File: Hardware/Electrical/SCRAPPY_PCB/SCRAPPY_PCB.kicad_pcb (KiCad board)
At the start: 2 copper layers, 87.6 x 96.5 mm, 54 parts, among them J1 Screw_Terminal_01x02, J2 Conn_01x04, J3 Conn_01x03, J4 Conn_01x03, J5 Conn_01x03, J6 Conn_01x04, J7 Conn_01x04, J8 Conn_01x04, J9 Conn_01x04, Q1 PN2222A, Q2 PN2222A, Q3 PN2222A, U1 ESP32-DevBoard, U2 L7805, U3 LM324

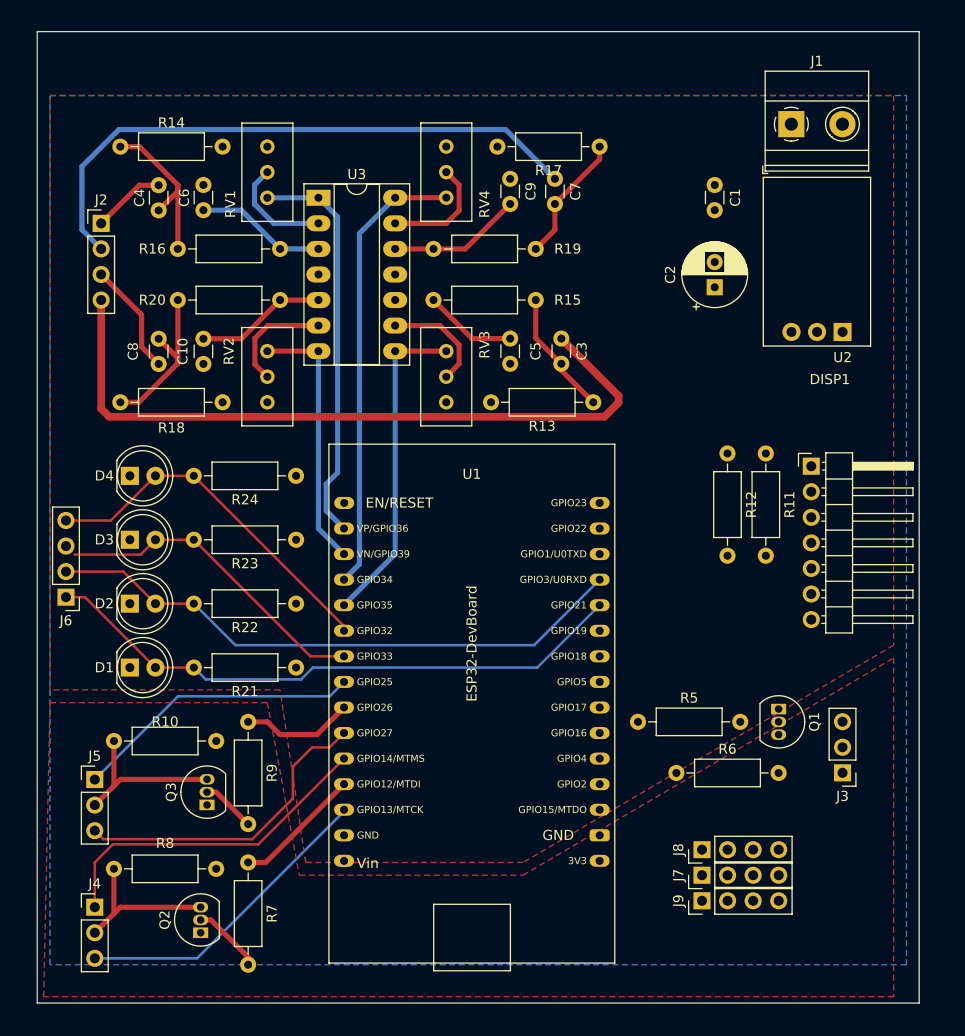
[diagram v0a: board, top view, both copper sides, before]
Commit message: Updated PCB; Ready for Manufacture
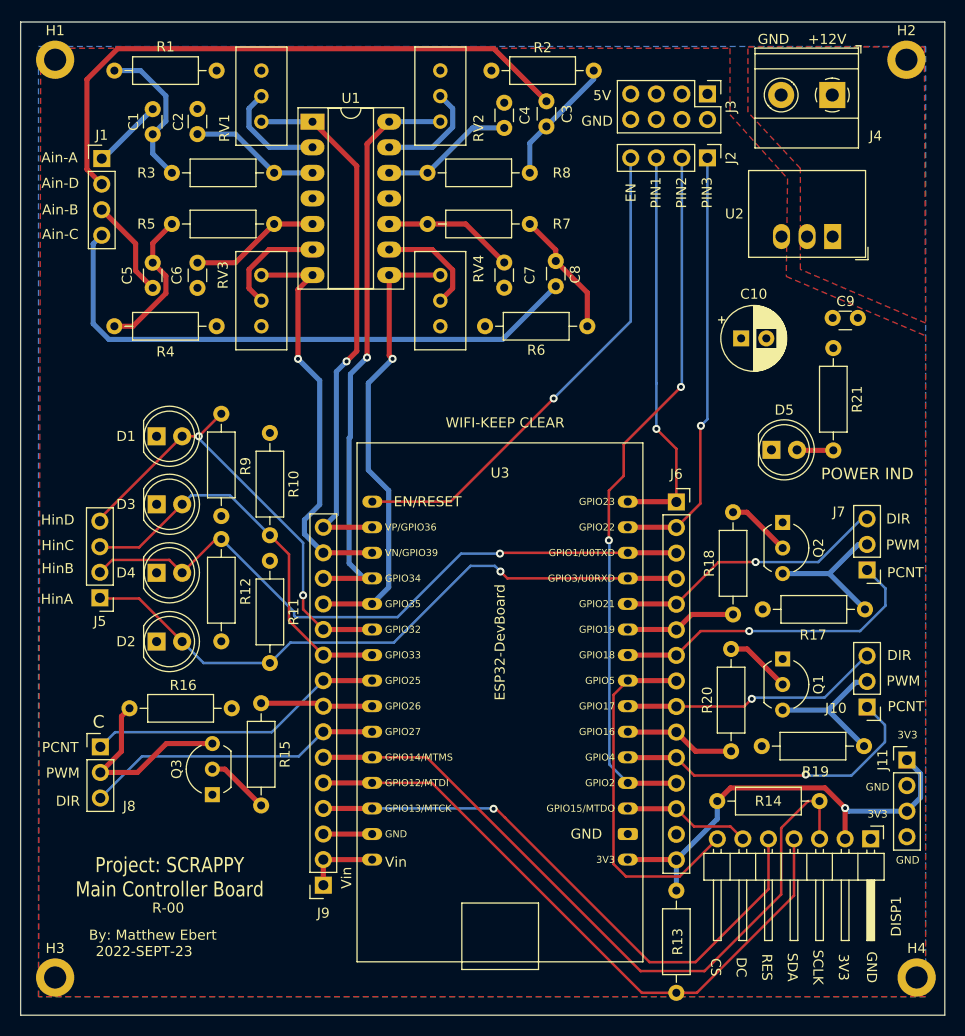
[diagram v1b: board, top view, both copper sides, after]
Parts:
- removed the J7 at (115.6, 133.3)
- added D5: LED, LED_THT:LED_D5.0mm_Clear, F.Cu at (122.5, 91.1)
- added H1: MountingHole, MountingHole:MountingHole_2.2mm_M2_DIN965_Pad, F.Cu at (51.3, 52.3)
- added H2: MountingHole, MountingHole:MountingHole_2.2mm_M2_DIN965_Pad, F.Cu at (135.9, 52.3)
- added H3: MountingHole, MountingHole:MountingHole_2.2mm_M2_DIN965_Pad, F.Cu at (51.3, 143.5)
- added H4: MountingHole, MountingHole:MountingHole_2.2mm_M2_DIN965_Pad, F.Cu at (136.9, 143.5)
- added J11: Conn_02x02_Odd_Even, Connector_PinHeader_2.54mm:PinHeader_1x04_P2.54mm_Vertical, F.Cu at (135.9, 121.9)
- added J3: Conn_02x04_Counter_Clockwise, Connector_PinHeader_2.54mm:PinHeader_2x04_P2.54mm_Vertical, F.Cu at (116.1, 55.7)
- added J6: Conn_01x15, Connector_PinSocket_2.54mm:PinSocket_1x15_P2.54mm_Vertical, F.Cu at (113.0, 96.3)
- added R21: R, Resistor_THT:R_Axial_DIN0207_L6.3mm_D2.5mm_P10.16mm_Horizontal, F.Cu at (128.6, 81.0)
- J9: value Conn_01x04 -> Conn_01x15; footprint Connector_PinHeader_2.54mm:PinHeader_1x04_P2.54mm_Vertical -> Connector_PinSocket_2.54mm:PinSocket_1x15_P2.54mm_Vertical
- Q1, Q2, Q3: footprint Package_TO_SOT_THT:TO-92_Inline -> Package_TO_SOT_THT:TO-92_Inline_Wide
- U2: footprint Converter_DCDC:Converter_DCDC_Murata_OKI-78SR_Horizontal -> Converter_DCDC:Converter_DCDC_RECOM_R-78B-2.0_THT
- moved J7 83.7 mm to (132.0, 103.0), turned to 180 degrees
- moved Q2 70.8 mm to (123.6, 98.3), turned to -90 degrees
- moved J2 68.7 mm to (116.1, 62.1), turned to -90 degrees
- moved R17 60.1 mm to (121.6, 106.9), turned to 0 degrees
- moved R18 54.1 mm to (118.7, 107.4), turned to 90 degrees
- moved R13 44.3 mm to (113.0, 134.9)
- moved J9 37.7 mm to (78.0, 134.3), turned to 180 degrees
- moved DISP1 37.5 mm to (132.3, 129.7), turned to -90 degrees
- moved R14 34.6 mm to (117.1, 126.0), turned to 0 degrees
- moved C9 19.6 mm to (131.1, 78.2), turned to 180 degrees
- moved R10 10.9 mm to (72.6, 89.4), turned to -90 degrees
- moved R11 10.9 mm to (72.6, 102.1), turned to -90 degrees
- moved R20 9.70 mm to (118.5, 121.0), turned to 90 degrees
- moved U2 9.53 mm to (128.6, 69.9)
- moved R19 8.90 mm to (121.5, 120.5)
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- renumbered C4 to C1, C2 to C10, C6 to C2, C7 to C3, C9 to C4, C8 to C5, C10 to C6, C5 to C7, C3 to C8, C1 to C9, D4 to D1, D1 to D2, D2 to D4, J2 to J1, J3 to J10, J8 to J2, J1 to J4, J6 to J5, J4 to J7, J5 to J8, R14 to R1, R23 to R10, R21 to R11, R22 to R12, R11 to R13, R12 to R14, R9 to R15, R10 to R16, R8 to R17, R7 to R18, R6 to R19, R17 to R2, R5 to R20, R16 to R3, R18 to R4, R20 to R5, R13 to R6, R15 to R7, R19 to R8, R24 to R9, RV4 to RV2, RV2 to RV3, RV3 to RV4, U3 to U1, U1 to U3
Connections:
- C9 pad 2: +12V -> +5V
- J2 pad 1: /PIN_1 -> /PIN_3
- J2 pad 3: /PIN_3 -> /PIN_1
- J9 pad 1: GND -> +5V
- J9 pad 2: GND -> +5V
- J9 pad 4: GND -> /RES
- R11 pad 1: +5V -> unconnected-(R11-Pad1)
- R16 pad 1: +3V3 -> +5V
- R17 pad 1: +3V3 -> +5V
- R19 pad 1: +3V3 -> +5V
- U3 pad 11: /PCNT_B -> /SCLK
- U3 pad 12: /PWM_B -> /SDA
- U3 pad 13: /DIR_B -> /RES
- U3 pad 18: /PIN_1 -> /DC
- U3 pad 24: /SCLK -> /PCNT_B
- U3 pad 25: /SDA -> /PWM_B
- U3 pad 26: /HALL-IN_A -> /DIR_B
- U3 pad 27: /HALL-IN_B -> /HALL-IN_A
- U3 pad 28: /PIN_3 -> /HALL-IN_B
- U3 pad 29: /RES -> /PIN_3
- U3 pad 30: /DC -> /PIN_1
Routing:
- net /SCLK: track 0.00 -> 72.7 mm
- net /PIN_2: track 0.00 -> 70.7 mm, vias 0 -> 2
- net /SDA: track 0.00 -> 65.0 mm
- net /RES: track 0.00 -> 58.6 mm, vias 0 -> 1
- net Net-(J2-Pad4): track 0.00 -> 49.3 mm, vias 0 -> 1
- net +3V3: track 0.00 -> 45.0 mm, vias 0 -> 1
- net /PIN_3: track 0.00 -> 42.8 mm, vias 0 -> 1
- net /PIN_1: track 0.00 -> 39.9 mm, vias 0 -> 1
- net /CS: track 0.00 -> 36.0 mm
- net /PCNT_A: track 0.00 -> 32.0 mm, vias 0 -> 1
- net /DIR_A: track 0.00 -> 25.9 mm, vias 0 -> 1
- net /INV_PWM_A: track 0.00 -> 14.6 mm
- net /Aout_B: track 26.3 -> 40.4 mm, vias 0 -> 1
- net /Ain_C: track 71.8 -> 57.9 mm
- net /Aout_A: track 39.9 -> 53.4 mm, vias 0 -> 1
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- added copper zone on F.Cu, net +12V
- removed copper zone on F.Cu, net +3V3
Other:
- board size 87.6 x 96.5 mm -> 91.8 x 98.7 mm
- board text added: "+12V"
- board text added: "2022-SEPT-23"
- board text added: "3V3"
- board text added: "5V"
- board text added: "Ain-A"
- board text added: "Ain-B"
- board text added: "Ain-C"
- board text added: "Ain-D"
- board text added: "By: Matthew Ebert"
- board text added: "C"
- board text added: "CS"
- board text added: "DC"
- board text added: "DIR"
- board text added: "EN"
- board text added: "GND"
- board text added: "HinA"
- board text added: "HinB"
- board text added: "HinC"
- board text added: "HinD"
- board text added: "PCNT"
- board text added: "PIN1"
- board text added: "PIN2"
- board text added: "PIN3"
- board text added: "POWER IND"
- board text added: "PWM"
- board text added: "Project: SCRAPPY Main Controller Board"
- board text added: "R-00"
- board text added: "RES"
- board text added: "SCLK"
- board text added: "SDA"
- board text added: "Vin"
- board text added: "WIFI-KEEP CLEAR"
